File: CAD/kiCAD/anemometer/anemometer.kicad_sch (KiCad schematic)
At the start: 2 parts

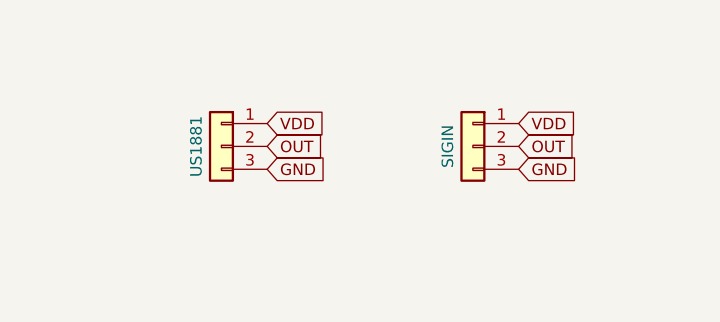
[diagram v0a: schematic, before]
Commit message: Update Schematics
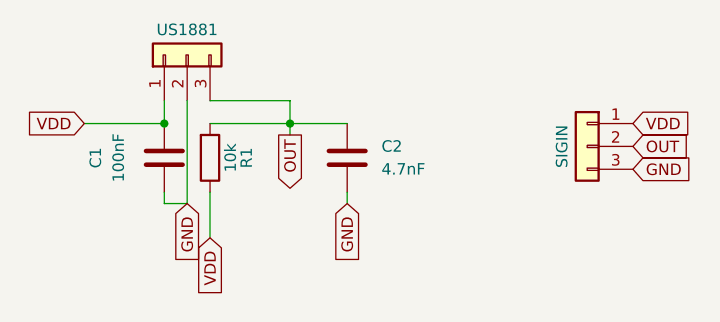
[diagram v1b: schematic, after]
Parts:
- added C1: 100nF, symbol Device:C
- added C2: 4.7nF, symbol Device:C
- added R1: 10k, symbol Device:R
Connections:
- net GND: now also US1881.2 (Pin_2), C1.1, C2.1; no longer US1881.3 (Pin_3)
- net OUT: now also US1881.3 (Pin_3), C2.2, R1.2; no longer US1881.2 (Pin_2)
- net VDD: now also C1.2, R1.1
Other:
- moved on the sheet: SIGIN, US1881
